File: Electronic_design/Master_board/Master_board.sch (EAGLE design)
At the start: 23 parts

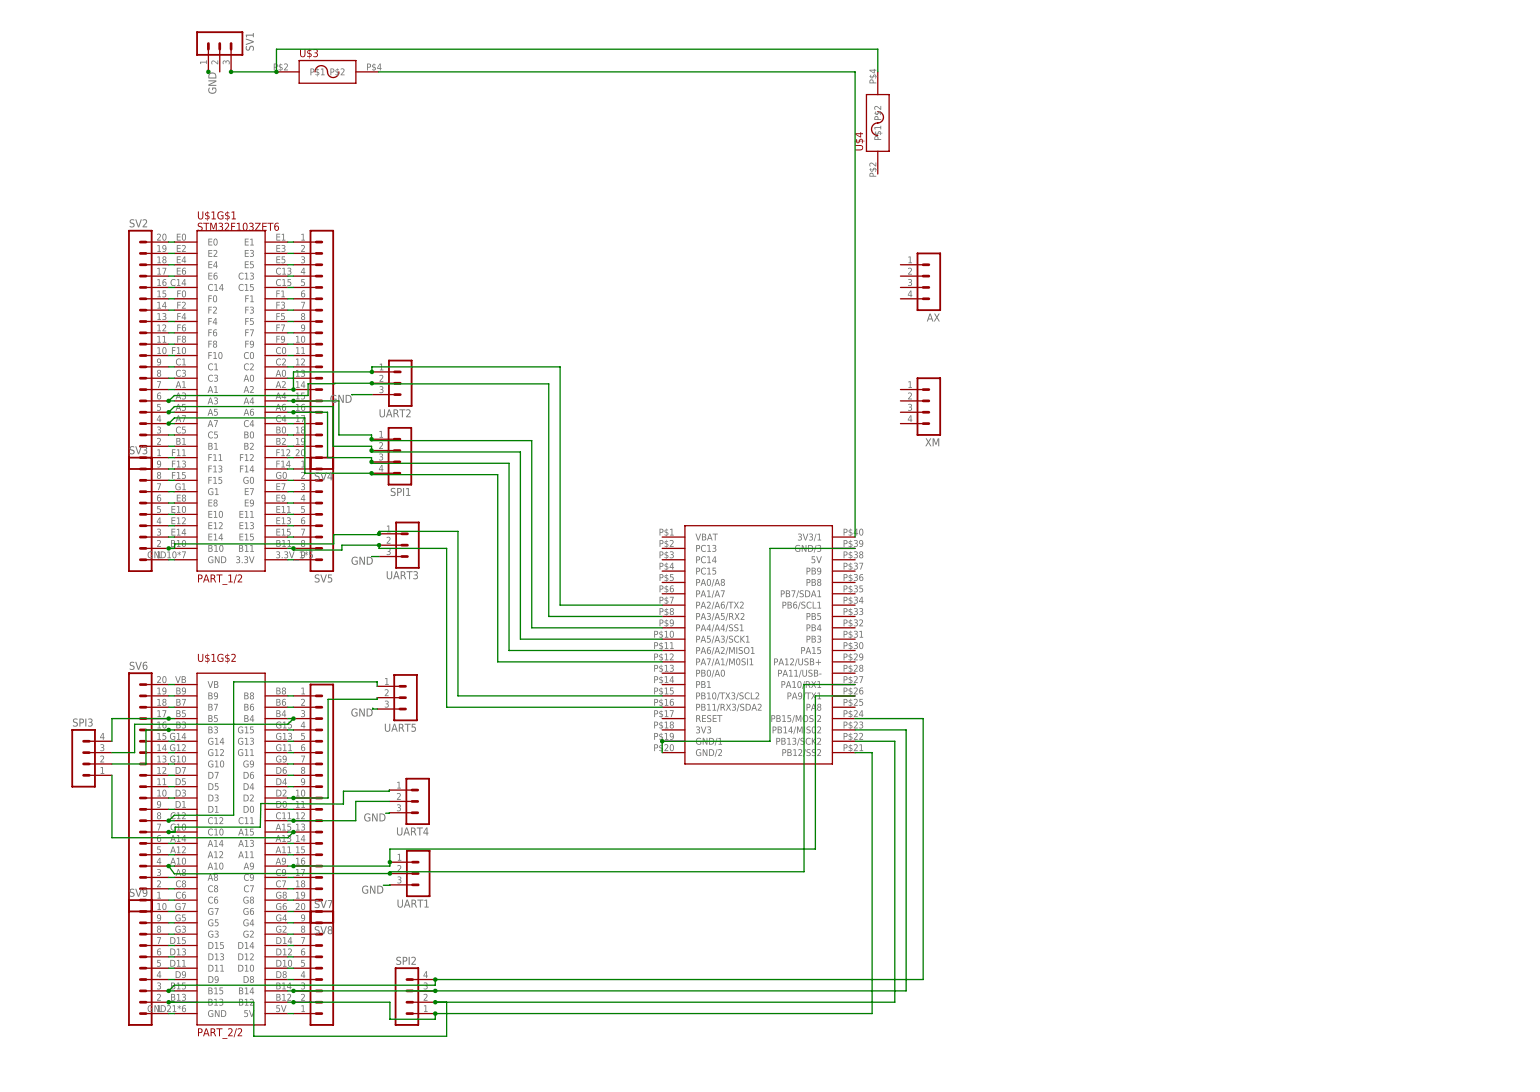
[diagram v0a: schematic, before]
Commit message: routage
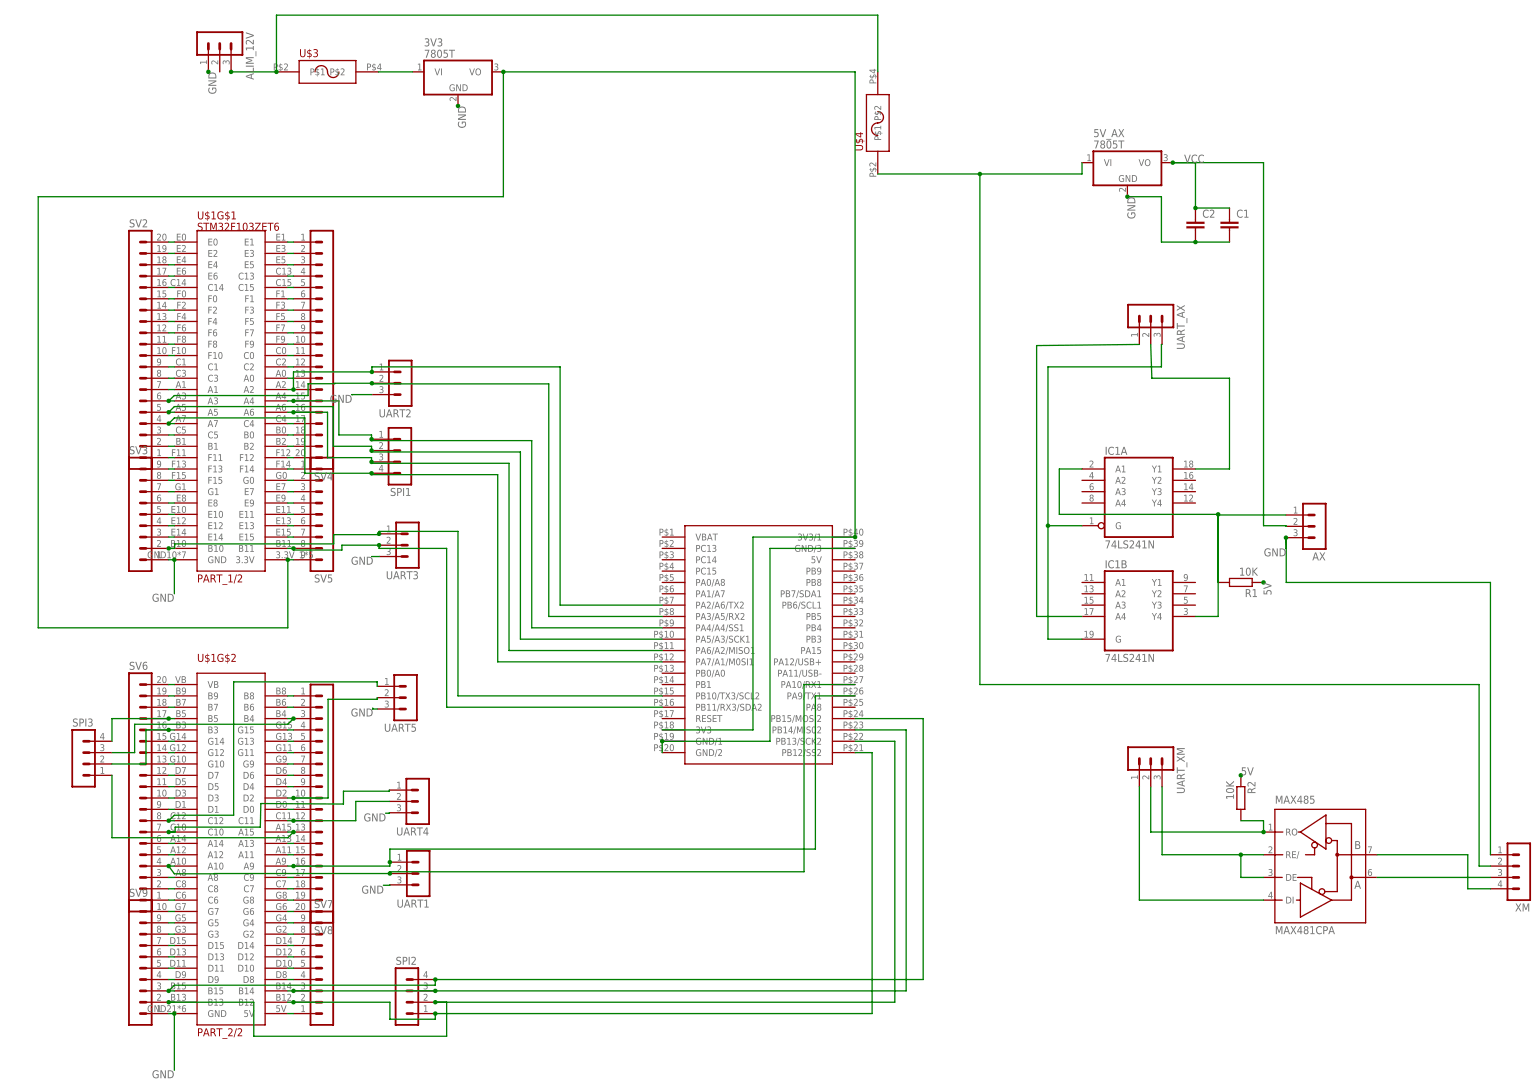
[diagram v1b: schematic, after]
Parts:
- added 3V3, 5V_AX: 7805T, linear:7805T
- added C1, C2: (no value), rcl:C-EU025-024X044
- added IC1: 74LS241N, 74xx-eu:74LS241N
- added MAX485: MAX481CPA, maxim:MAX481CPA
- added R1, R2: 10K, rcl:R-EU_0309/12
- added UART_AX, UART_XM: (no value), con-lstb:MA03-1
- AX: device con-lstb:MA04-1 -> con-lstb:MA03-1
- renumbered SV1 to ALIM_12V
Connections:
- net N$2 renamed VIN
- removed net N$113: SV9.1, U$1G$2.GND
- removed net N$43: SV3.1, U$1G$1.GND
- removed net N$75: SV5.9, U$1G$1.3.3V
- new net 12V: 5V_AX.VI, U$4.P$1, XM.2
- new net 5V: R1.1, R2.1
- new net CTRL_AX: IC1A.G, IC1B.G, UART_AX.3
- new net CTRL_XM: MAX485G$1.DE, MAX485G$1.RE/, UART_XM.3
- new net D+: MAX485G$1.A, XM.3
- new net D-: MAX485G$1.B, XM.4
- new net DATA_AX: AX.1, IC1A.A1, IC1B.Y4, R1.2
- new net N$121: 3V3.VI, U$3.P$2
- new net RX_AX: IC1A.Y1, UART_AX.2
- new net RX_XM: MAX485G$1.RO, R2.2, UART_XM.2
- new net TX_AX: IC1B.A4, UART_AX.1
- new net TX_XM: MAX485G$1.DI, UART_XM.1
- new net VCC: 5V_AX.VO, AX.2, C1.1, C2.1
- net GND: now also 3V3.GND, 5V_AX.GND, AX.3, C1.2, C2.2, SV3.1, SV9.1, U$1G$1.GND, U$1G$2.GND, XM.1
- net N$1: now also 3V3.VO, SV5.9, U$1G$1.3.3V, U$2.3V3; no longer U$3.P$2
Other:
- moved on the sheet: XM

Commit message: ameliorations
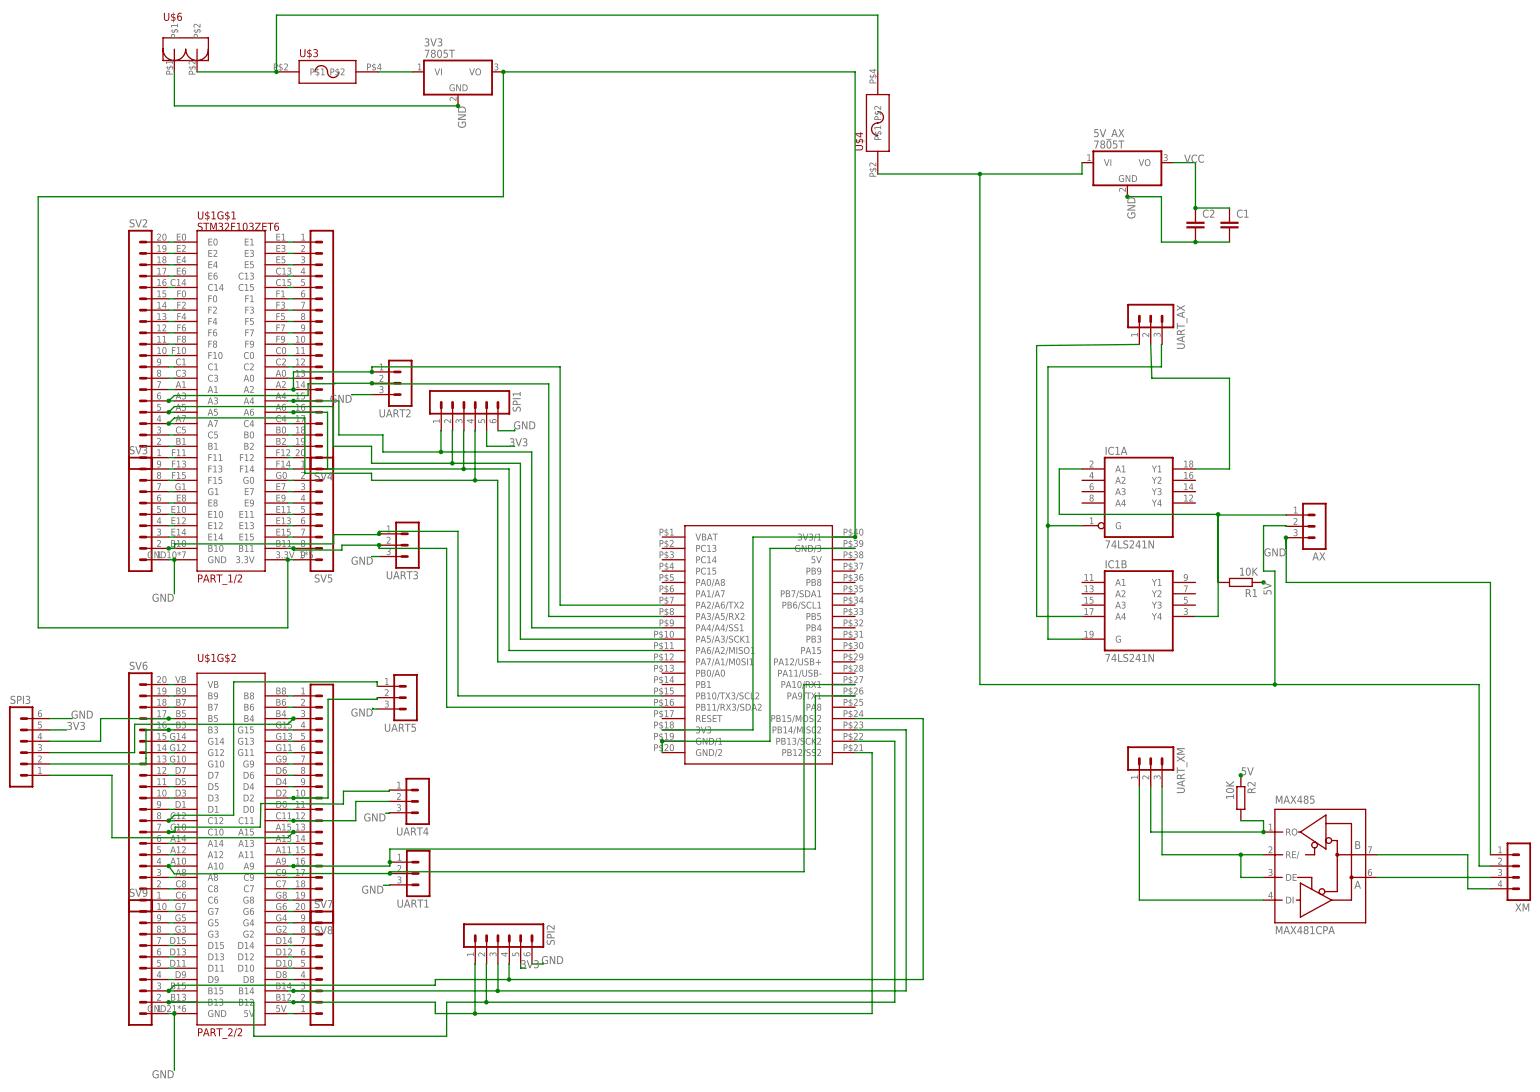
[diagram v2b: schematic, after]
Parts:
- removed ALIM_12V: (no value), con-lstb:MA03-1
- added U$6: GREEN_HEADER, PowerHeaders:GREEN_HEADER
- SPI1, SPI2, SPI3: device con-lstb:MA04-1 -> con-lstb:MA06-1
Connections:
- net N$10 renamed TX4
- net N$11 renamed RX4
- net N$12 renamed RX5
- net N$13 renamed TX5
- net N$14 renamed NSS1
- net N$15 renamed SCK1
- net N$16 renamed MISO1
- net N$17 renamed MOSI1
- net N$18 renamed NSS2
- net N$19 renamed MISO2
- net N$20 renamed SCK2
- net N$21 renamed MOSI2
- net N$22 renamed NSS3
- net N$23 renamed SCK3
- net N$24 renamed MISO3
- net N$25 renamed MOSI3
- net N$28 renamed TX1
- net N$4 renamed TX2
- net N$5 renamed RX2
- net N$7 renamed RX1
- net N$8 renamed TX3
- net N$9 renamed RX3
- removed net N$1: 3V3.VO, SV5.9, U$1G$1.3.3V, U$2.3V3, U$2.3V3/1
- removed net N$3: U$2.GND/1, U$2.GND/2, U$2.GND/3
- new net 3V3: 3V3.VO, SPI1.5, SPI2.5, SPI3.5, SV5.9, U$1G$1.3.3V, U$2.3V3, U$2.3V3/1
- net 12V: now also AX.2
- net GND: now also SPI1.6, SPI2.6, SPI3.6, U$2.GND/1, U$2.GND/2, U$2.GND/3, U$6.P$1; no longer ALIM_12V.1
- net VCC: no longer AX.2
- net VIN: now also U$6.P$2; no longer ALIM_12V.3
